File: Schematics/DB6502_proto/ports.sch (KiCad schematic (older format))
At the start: 20 parts, among them J1 Power plug, J10 System Bus, J2 Controls, J3 AVR ISP, J4 Debug USB, J5 JPR, J6 Debug UART, J7 UART A, J8 UART B, J9 I/O Bus

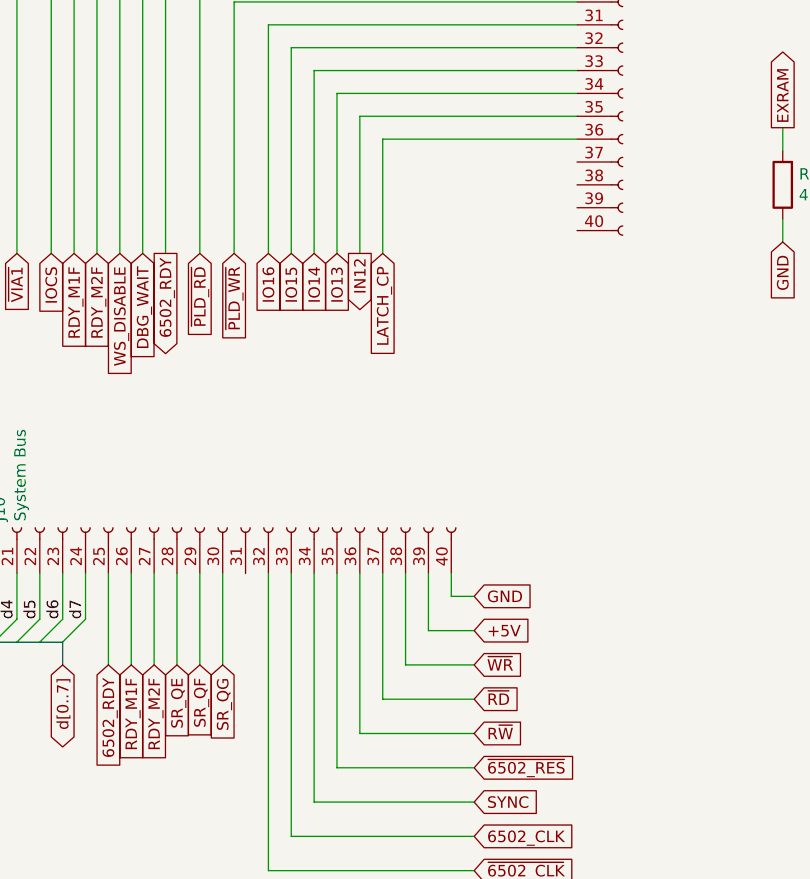
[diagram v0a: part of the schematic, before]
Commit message: Added one last line to the system
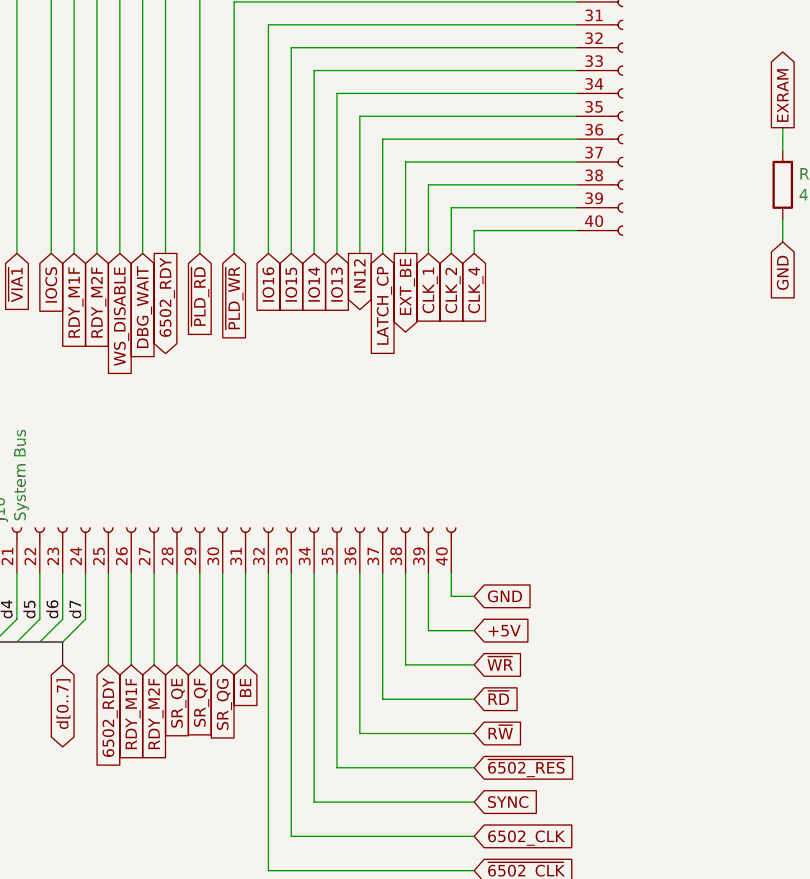
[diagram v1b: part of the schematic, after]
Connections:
- net BE: now also J10.31 (Pin_31)
- net CLK_1: now also J2.38 (Pin_38)
- net CLK_2: now also J2.39 (Pin_39)
- net CLK_4: now also J2.40 (Pin_40)
- net EXT_BE: now reaches J2.37 (Pin_37)
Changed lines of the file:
@@
 Wire Wire Line
 	5300 6800 5300 6400
+Text GLabel 6200 5000 3    50   Input ~ 0
+CLK_1
+Text GLabel 6300 5000 3    50   Input ~ 0
+CLK_2
+Text GLabel 6400 5000 3    50   Input ~ 0
+CLK_4
+Wire Wire Line
+	6400 5000 6400 4900
+Wire Wire Line
+	6400 4900 6850 4900
+Wire Wire Line
+	6300 5000 6300 4800
+Wire Wire Line
+	6300 4800 6850 4800
+Wire Wire Line
+	6200 5000 6200 4700
+Wire Wire Line
+	6200 4700 6850 4700
+Wire Wire Line
+	6100 5000 6100 4600
+Wire Wire Line
+	6100 4600 6850 4600
+Text GLabel 6100 5000 3    50   Output ~ 0
+EXT_BE
+Text GLabel 5400 6800 3    50   Input ~ 0
+BE
+Wire Wire Line
+	5400 6800 5400 6400
 Wire Bus Line
 	10750 2150 10750 2350
